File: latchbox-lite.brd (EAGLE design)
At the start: 59.1 x 21.8 mm, 28 parts, among them IC1 PIC12F1822SO08

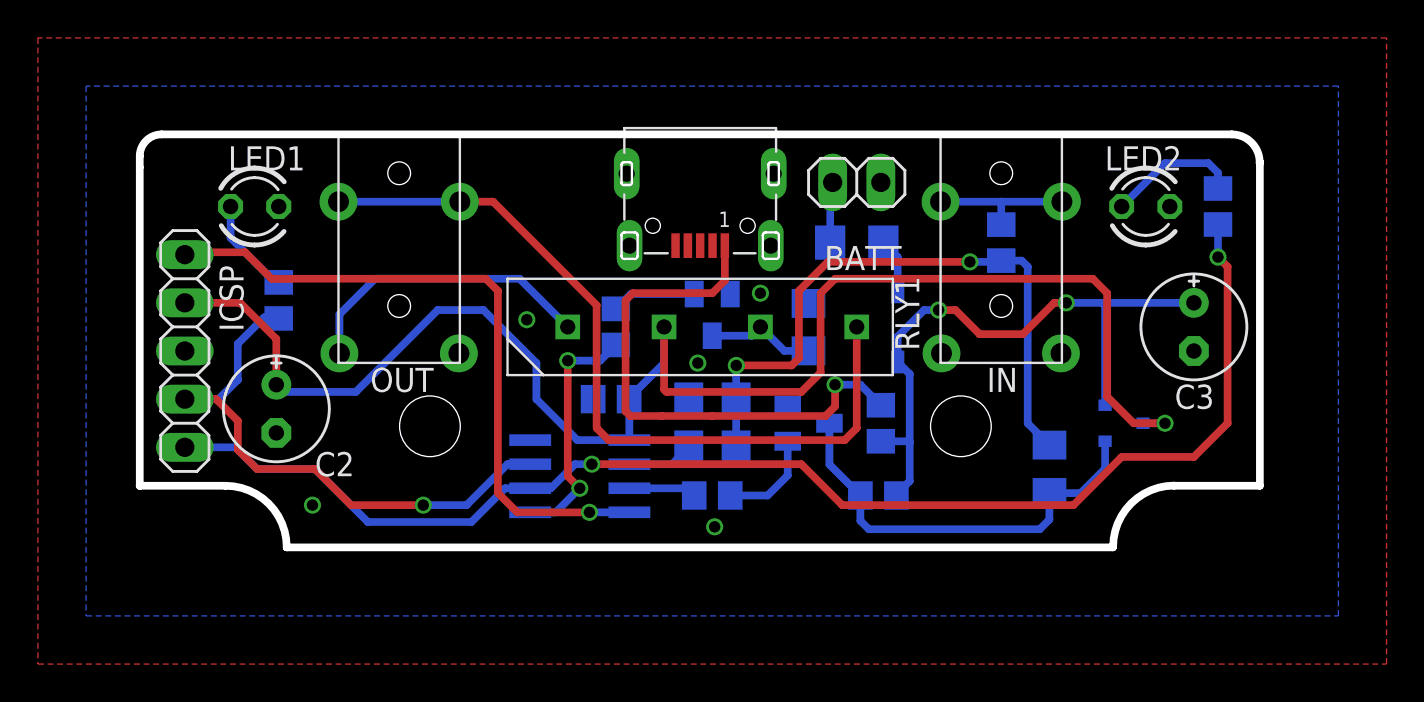
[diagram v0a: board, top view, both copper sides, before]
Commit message: v2 possible
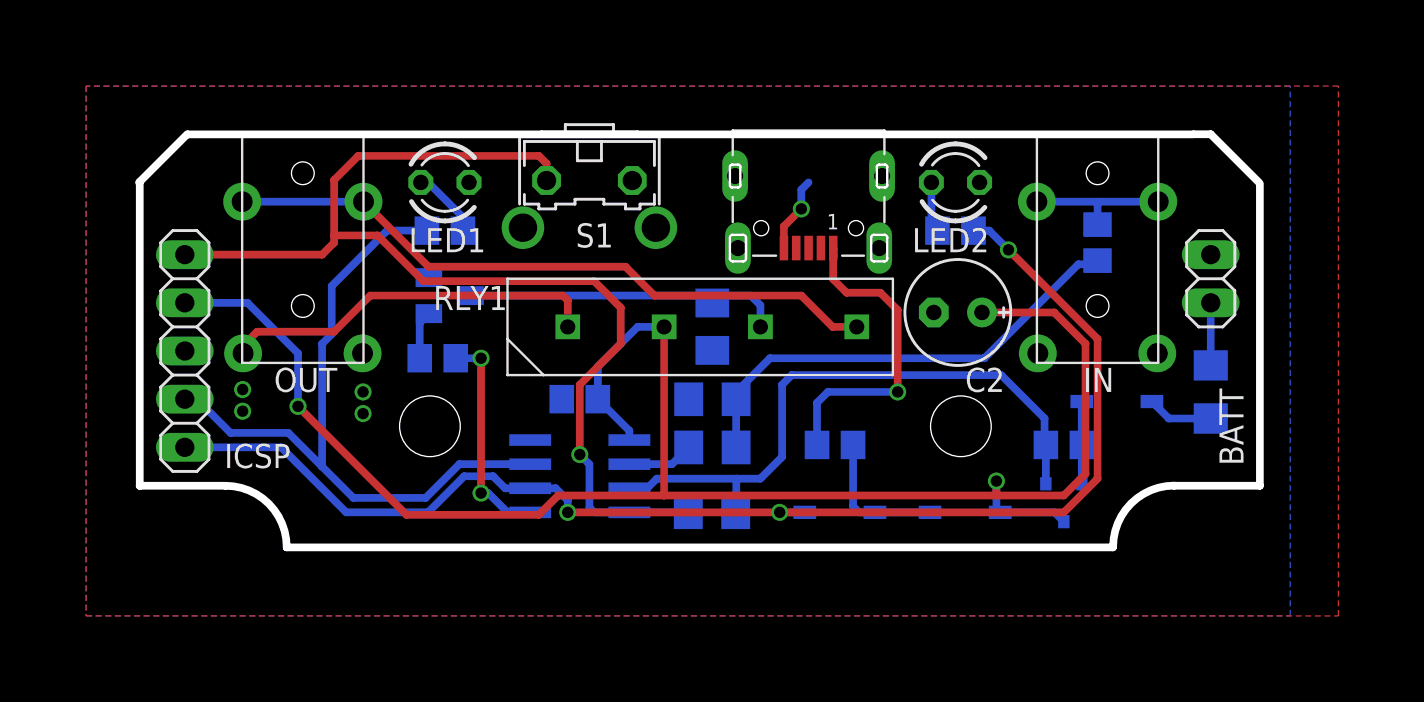
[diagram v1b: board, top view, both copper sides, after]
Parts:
- removed C3: (no value), rcl:E2,5-6E
- removed Q3: (no value), transistor:SOT23-BEC
- removed R7: 1k, rcl:R0805
- added D6, D7: 0805DIODE, jasons_stuff:0805DIODE
- added S1: (no value), switch-omron:B3F-31XX
- C2: value (none) -> 4u7
- D1, D3: value 0805DIODE -> (none); device jasons_stuff:0805DIODE -> microbuilder:SOD-123
- R1: value 1k -> 100r
- R2: value 100r -> 1k
- R3: value (none) -> 10k
- R4: value 10k -> 4r7
- R5: value (none) -> 1k
- moved C2 36.3 mm to (46.0, 23.6), turned to 180 degrees
- moved F1 20.3 mm to (59.3, 19.4), turned to 270 degrees
- moved Q2 20.1 mm to (19.2, 24.5)
- moved BATT 19.3 mm to (59.3, 25.4), turned to 270 degrees
- moved R5 16.2 mm to (18.5, 21.2)
- moved D2 10.4 mm to (46.4, 13.1), turned to 0 degrees
- moved R6 10.3 mm to (18.9, 27.9), turned to 0 degrees
- moved LED2 10.1 mm to (45.8, 30.5)
- moved LED1 10.1 mm to (18.9, 30.5)
- moved D3 9.92 mm to (39.8, 13.1), turned to 180 degrees
- moved R3 9.72 mm to (51.6, 16.6), turned to 180 degrees
- moved R1 6.63 mm to (53.3, 27.3)
- moved D4 5.97 mm to (33.0, 13.1), turned to 180 degrees
- moved USB 5.72 mm to (38.1, 28.1)
- moved Q1 5.26 mm to (51.6, 13.6), turned to 180 degrees
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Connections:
- removed net N: D1.C, Q1.1, Q2.C, R4.1
- removed net N$2: Q2.B, R5.1
- new net USB_POWER: D2.A, D3.A, R4.1
- net GND: now also D6.C, D7.C, S1.1; no longer C3.-, D3.C, D4.C, Q3.E
- net N$1: now also R1.1; no longer R2.1
- net N$10: now also R6.1; no longer R7.1
- net N$11: now also R6.2; no longer R7.2
- net N$12: now also D3.C, R2.2; no longer R1.2
- net N$14: now also D4.A, S1.2
- net N$15: now also D1.A; no longer D2.A
- net N$16: now also R4.2; no longer R3.2
- net N$3: now also R2.1; no longer R1.1
- net N$4: now also D1.C, R3.2; no longer C3.+, D2.C, R3.1, R4.2
- net N$6: now also Q2.B, R5.2; no longer Q3.B, R6.2
- net N$9: now also D7.A, Q2.C; no longer D3.A, Q3.C
- net OUTPUT: now also R5.1; no longer R6.1
- net POWER_CTRL: now also D4.C, Q1.1, R3.1; no longer R5.2
- net VCC: now also D2.C
- net Z: now also D6.A, R1.2; no longer D1.A, D4.A, R2.2
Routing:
- net POWER_CTRL: track 3.58 -> 32.9 mm
- net N$4: track 33.4 -> 4.46 mm, vias 2 -> 0
- net N: track 22.5 -> 0.00 mm
- net N$14: track 35.4 -> 57.9 mm
- net N$16: track 28.7 -> 16.8 mm
- net N$9: track 5.79 -> 17.0 mm
- net VCC: track 81.5 -> 91.5 mm, vias 1 -> 2
- net Z: track 34.1 -> 24.8 mm, vias 2 -> 0
- net USB_POWER: track 0.00 -> 7.43 mm
- net N$11: track 30.2 -> 37.1 mm, vias 1 -> 0
- net N$7: track 41.9 -> 35.1 mm
- net N$2: track 5.27 -> 0.00 mm
- net N$3: track 7.07 -> 2.67 mm
- net N$8: track 15.9 -> 20.1 mm
- net GND: track 0.51 -> 4.00 mm
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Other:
- outline, holes or cut-outs redrawn
- board text added: "pcb rev 2"
- board text removed: "pcb rev 1"

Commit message: V3
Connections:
- net GND: now also IN.1; no longer IN.3
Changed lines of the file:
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@@
 <contactref element="D6" pad="C"/>
 <contactref element="BATT" pad="1"/>
-<contactref element="IN" pad="3"/>
 <contactref element="D7" pad="C"/>
 <contactref element="Q2" pad="E"/>
@@
 <vertex x="66.04" y="35.56"/>
 </polygon>
+<contactref element="IN" pad="1"/>
 </signal>
 <signal name="N$5">
